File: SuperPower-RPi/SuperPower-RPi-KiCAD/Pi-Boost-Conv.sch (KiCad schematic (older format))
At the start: 20 parts, among them U1 TPS61088

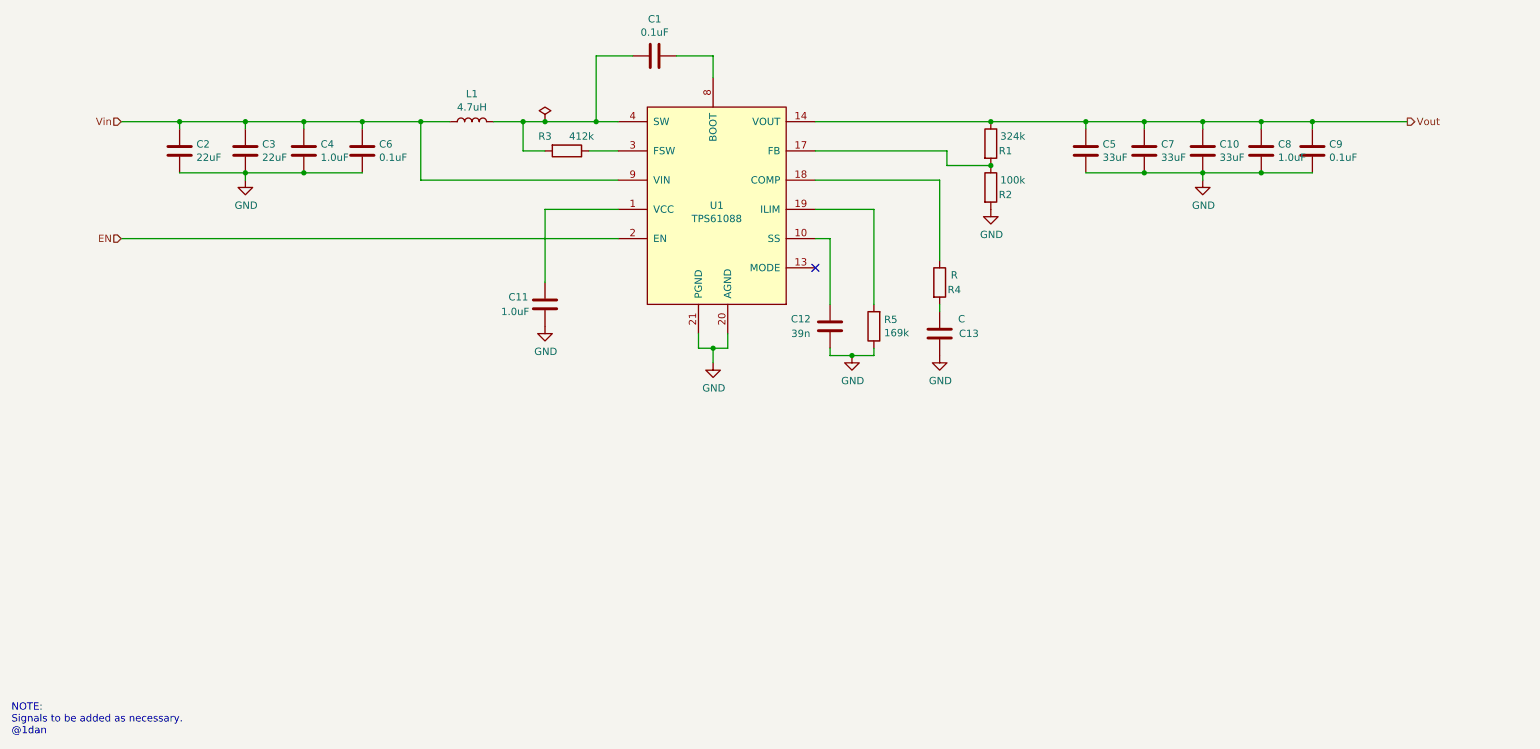
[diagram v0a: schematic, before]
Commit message: Updated components. Mostly caps and resistors.
(cherry picked from commit e921c80666429be92cc496d87bcbd557350196b5)
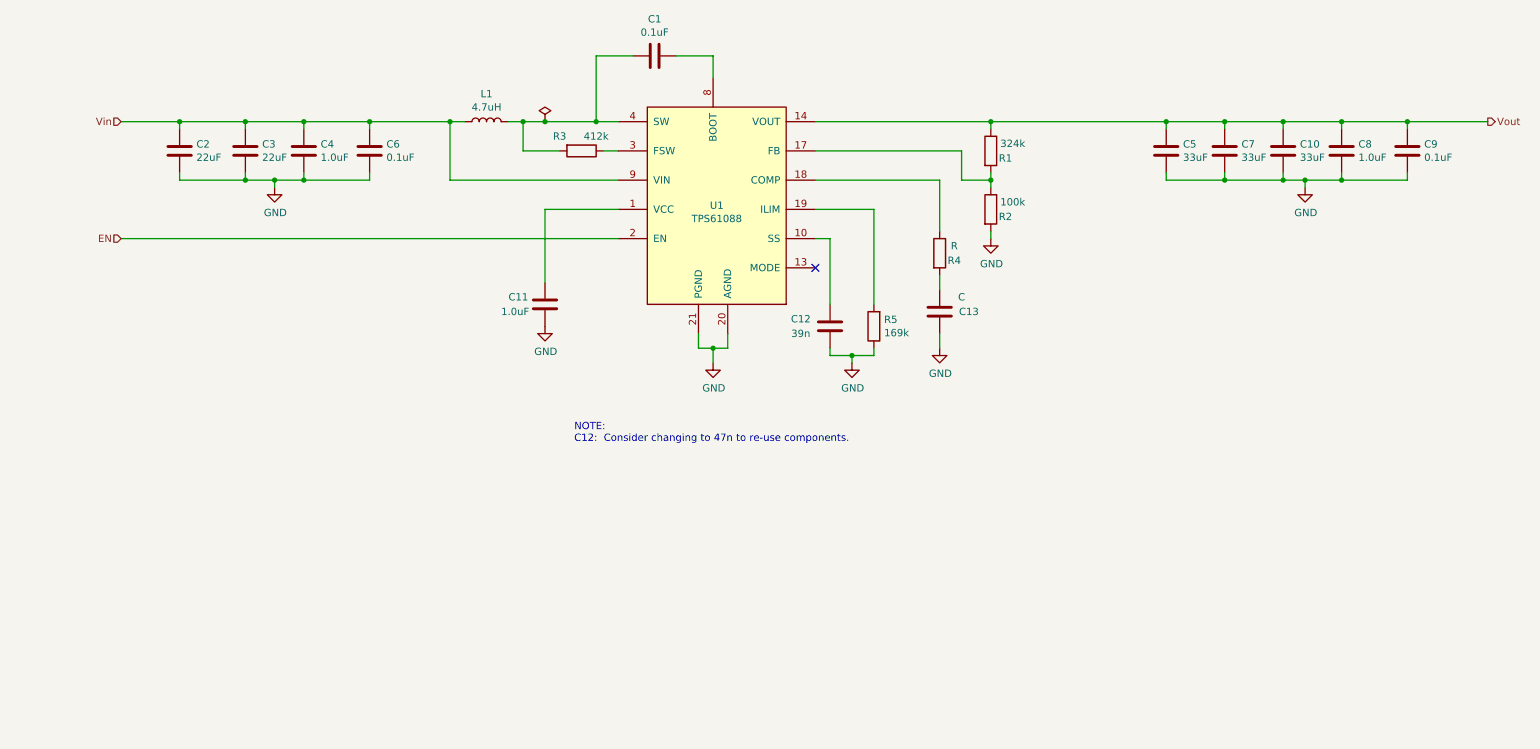
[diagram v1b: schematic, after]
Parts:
- C11, C4, C8: footprint (none) -> Capacitor_SMD:C_0603_1608Metric; Digi-Key PN (none) -> 1276-1184-1-ND; Mfg (none) -> Samsung; Mfg PN (none) -> CL10B105KA8NNNC
- C2, C3: footprint (none) -> Capacitor_SMD:C_1206_3216Metric; Digi-Key PN (none) -> 1276-3047-1-ND; Mfg (none) -> Samsung; Mfg PN (none) -> CL31A226KAHNNNE
- R2: Digi-Key PN (none) -> 311-100KHRCT-ND; Mfg (none) -> Yageo; Mfg PN (none) -> RC0603FR-07100KL
- R5: footprint (none) -> Resistor_SMD:R_0603_1608Metric
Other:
- note added: "NOTE:\nC12: Consider changing to 47n to re-use components."
- note removed: "NOTE:\nSignals to be added as necessary.\n@1dan"
- moved on the sheet: C10, C13, C5, C6, C7, C8, C9, L1, R1, R2, R3, R4
